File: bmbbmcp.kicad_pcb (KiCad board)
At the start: 4 copper layers, 57 x 14 mm, 20 parts, among them J1 USB_OTG, J2 ARM_SWD, J3 Conn_01x04_Socket, U1 MDBT50Q-1MV2, U2 AP2112K, Y1 32.768

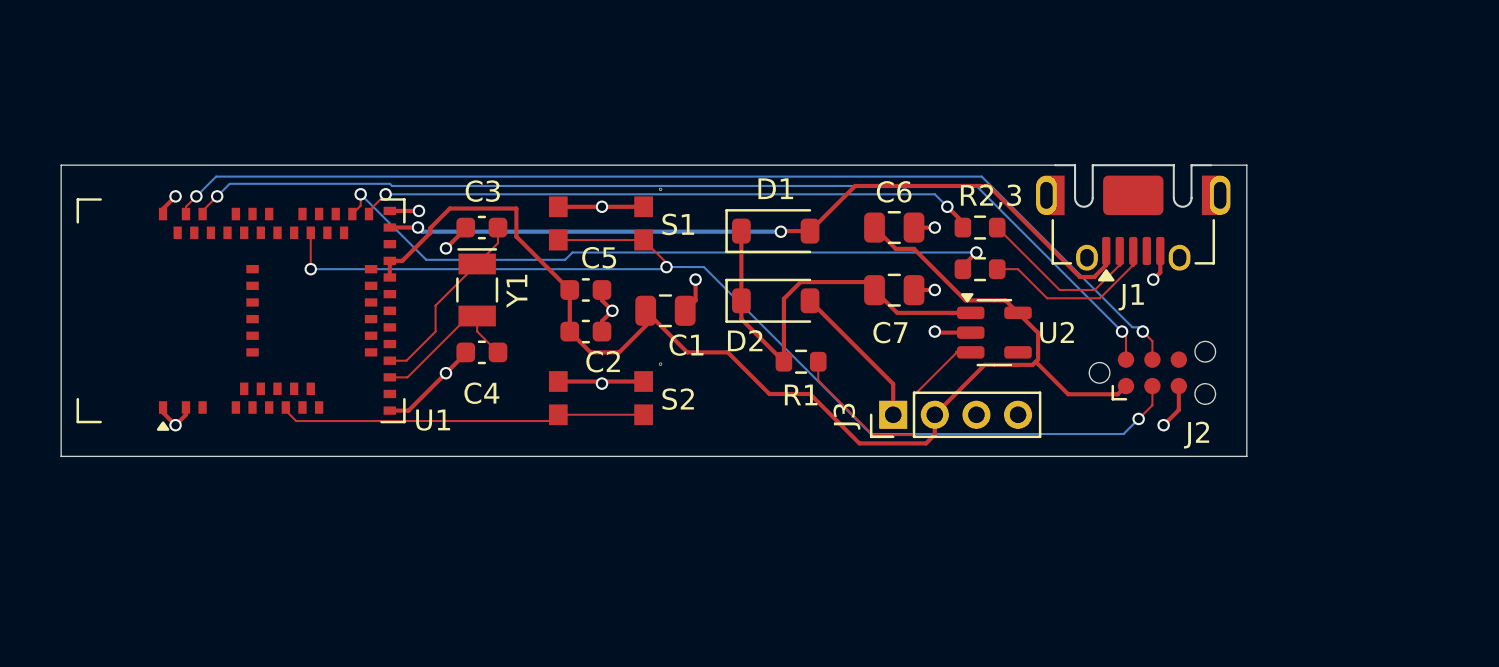
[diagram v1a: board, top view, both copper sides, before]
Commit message: Initial full board design
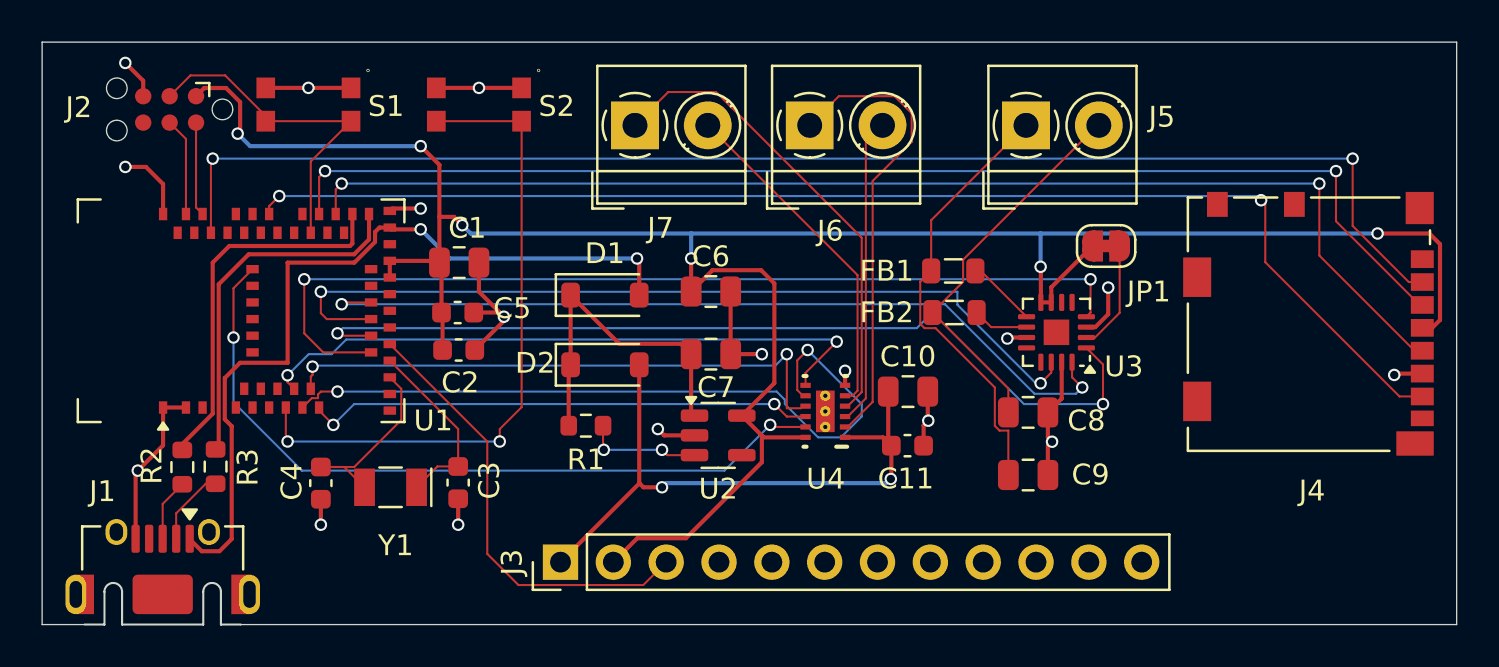
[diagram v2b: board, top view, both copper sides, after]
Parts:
- added C10: 10uF, Capacitor_SMD:C_0805_2012Metric, F.Cu at (160.6, 96.8)
- added C11: 0.1uF, Capacitor_SMD:C_0603_1608Metric, F.Cu at (160.6, 99.4)
- added C8: 220pF, Capacitor_SMD:C_0805_2012Metric, F.Cu at (166.4, 97.8)
- added C9: 220pF, Capacitor_SMD:C_0805_2012Metric, F.Cu at (166.4, 100.8)
- added FB1: FerriteBead, Inductor_SMD:L_0805_2012Metric, F.Cu at (162.8, 91.0)
- added FB2: FerriteBead, Inductor_SMD:L_0805_2012Metric, F.Cu at (162.9, 93.0)
- added J4: Micro_SD_Card, Connector_Card:microSD_HC_Molex_104031-0811, F.Cu at (179.9, 93.5)
- added J5: Screw_Terminal_01x02, TerminalBlock_MetzConnect:TerminalBlock_MetzConnect_Type059_RT06302HBWC_1x02_P3.50mm_Horizontal, F.Cu at (166.3, 84.0)
- added J6: Screw_Terminal_01x02, TerminalBlock_MetzConnect:TerminalBlock_MetzConnect_Type059_RT06302HBWC_1x02_P3.50mm_Horizontal, F.Cu at (155.9, 84.0)
- added J7: Screw_Terminal_01x02, TerminalBlock_MetzConnect:TerminalBlock_MetzConnect_Type059_RT06302HBWC_1x02_P3.50mm_Horizontal, F.Cu at (147.5, 84.0)
- added JP1: SolderJumper, Jumper:SolderJumper-2_P1.3mm_Bridged_RoundedPad1.0x1.5mm, F.Cu at (170.2, 89.8)
- added U3: MAX98357A, Package_DFN_QFN:TQFN-16-1EP_3x3mm_P0.5mm_EP1.23x1.23mm, F.Cu at (167.8, 94.0)
- added U4: DRV8835DSSR, DRV8835:DSS0012A, F.Cu at (156.6, 97.8)
- J2: value ARM_SWD -> Conn_ARM_SWD_TagConnect_TC2030
- J3: value Conn_01x04_Socket -> Conn_01x12_Socket; footprint Connector_PinHeader_2.00mm:PinHeader_1x04_P2.00mm_Vertical -> Connector_PinHeader_2.54mm:PinHeader_1x12_P2.54mm_Vertical
- U2: value AP2112K -> AP2112K-3.3
- moved J1 50.7 mm to (124.8, 106.9), turned to 0 degrees
- moved J2 48.9 mm to (125.1, 83.2), turned to 180 degrees
- moved R2 39.5 mm to (125.7, 100.4), turned to -90 degrees
- moved R3 38.5 mm to (127.3, 100.4), turned to -90 degrees
- moved J3 17.5 mm to (143.9, 105.0)
- moved S2 15.3 mm to (140.0, 83.0)
- moved S1 15.2 mm to (131.8, 83.0)
- moved U2 14.2 mm to (151.5, 98.9)
- moved C3 12.3 mm to (139.0, 101.2), turned to 90 degrees
- moved R1 10.8 mm to (145.1, 98.4)
- moved Y1 10.4 mm to (135.8, 101.4), turned to 180 degrees
- moved C1 10.2 mm to (139.1, 90.6)
- moved C4 9.97 mm to (132.4, 101.2), turned to 90 degrees
- moved C7 9.34 mm to (151.2, 95.0)
- moved C6 9.34 mm to (151.2, 92.0)
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- renumbered R2,3 to R3
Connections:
- J3 pad 3: unconnected-(J3-Pin_3-Pad3) -> /BTN1
- U1 pad 11: unconnected-(U1-P0.02-Pad11) -> /MOTOR_B2
- U1 pad 12: unconnected-(U1-P0.31-Pad12) -> /MOTOR_B1
- U1 pad 13: unconnected-(U1-P0.28-Pad13) -> /MOTOR_A2
- U1 pad 14: unconnected-(U1-P0.30-Pad14) -> /MOTOR_A1
- U1 pad 19: unconnected-(U1-P0.26-Pad19) -> /I2S_MODE
- U1 pad 20: unconnected-(U1-P0.04-Pad20) -> /BTN1
- U1 pad 21: unconnected-(U1-P0.05-Pad21) -> /I2S_DOUT
- U1 pad 23: unconnected-(U1-P0.07-Pad23) -> /I2S_LRCK
- U1 pad 25: unconnected-(U1-P1.08-Pad25) -> /I2S_SCK
- U1 pad 37: unconnected-(U1-P0.13-Pad37) -> /SPI_SCLK
- U1 pad 39: unconnected-(U1-P0.15-Pad39) -> /SPI_MOSI
- U1 pad 44: unconnected-(U1-P0.20-Pad44) -> /SPI_MISO
- U1 pad 50: unconnected-(U1-P1.02-Pad50) -> /SPI_CS1
- U1 pad 61: unconnected-(U1-P1.01-Pad61) -> /MOTOR_CTRL
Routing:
- net /SPI_CS1: track 0.00 -> 66.1 mm, vias 0 -> 2
- net /SPI_MISO: track 0.00 -> 61.6 mm, vias 0 -> 2
- net /SPI_MOSI: track 0.00 -> 59.0 mm, vias 0 -> 2
- net /SPI_SCLK: track 0.00 -> 58.9 mm, vias 0 -> 2
- net +3.3V: track 60.6 -> 115.7 mm, vias 0 -> 6
- net /SWCLK: track 51.8 -> 4.72 mm, vias 2 -> 0
- net /I2S_MODE: track 0.00 -> 45.9 mm, vias 0 -> 2
- net /SWDIO: track 49.3 -> 4.53 mm, vias 2 -> 0
- net /I2S_DOUT: track 0.00 -> 43.7 mm, vias 0 -> 2
- net /I2S_LRCK: track 0.00 -> 41.6 mm, vias 0 -> 2
- net /I2S_SCK: track 0.00 -> 40.4 mm, vias 0 -> 2
- net /MOTOR_CTRL: track 0.00 -> 36.6 mm, vias 0 -> 2
- net /~{RESET}: track 52.9 -> 16.4 mm, vias 3 -> 0
- net /MOTOR_B1: track 0.00 -> 35.7 mm, vias 0 -> 2
- net /MOTOR_B2: track 0.00 -> 30.8 mm, vias 0 -> 2
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- added copper zone on In1.Cu, net GND
- removed copper zone on In2.Cu, net GND
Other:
- board size 57 x 14 mm -> 68 x 28 mm
